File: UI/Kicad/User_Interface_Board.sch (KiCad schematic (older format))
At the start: 13 parts, among them J1 BHR-16-HUA, J2 Conn_01x02_Male, J3 Conn_01x02_Male, J4 Conn_01x02_Male, J5 Conn_01x02_Male, J6 Conn_01x08_Male, J7 Conn_01x05_Male, J8 Conn_01x03_Male

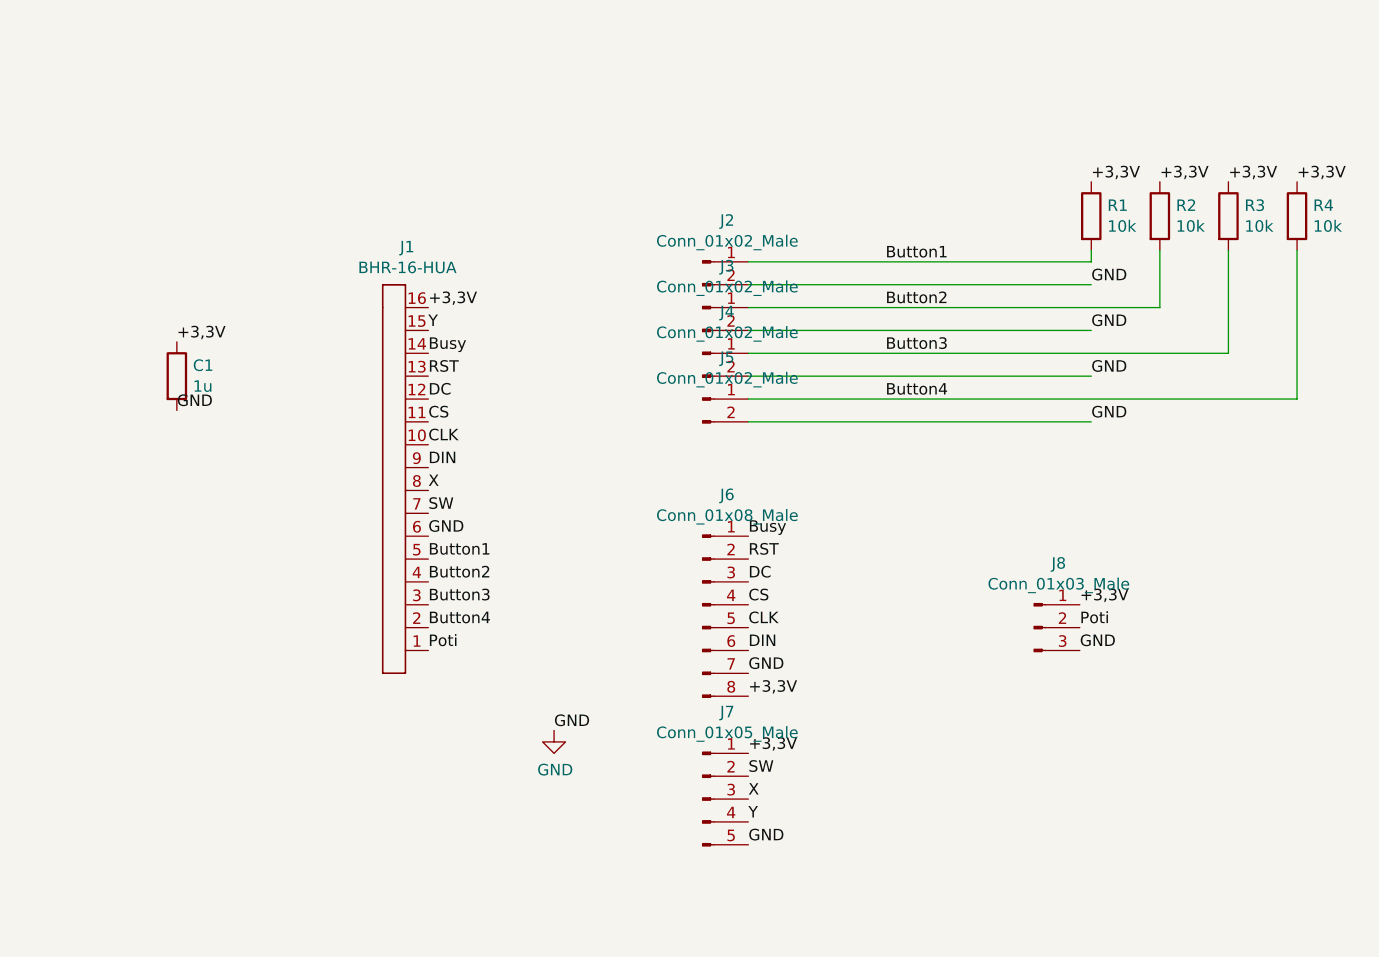
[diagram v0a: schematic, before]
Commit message: Display-Board Updated!
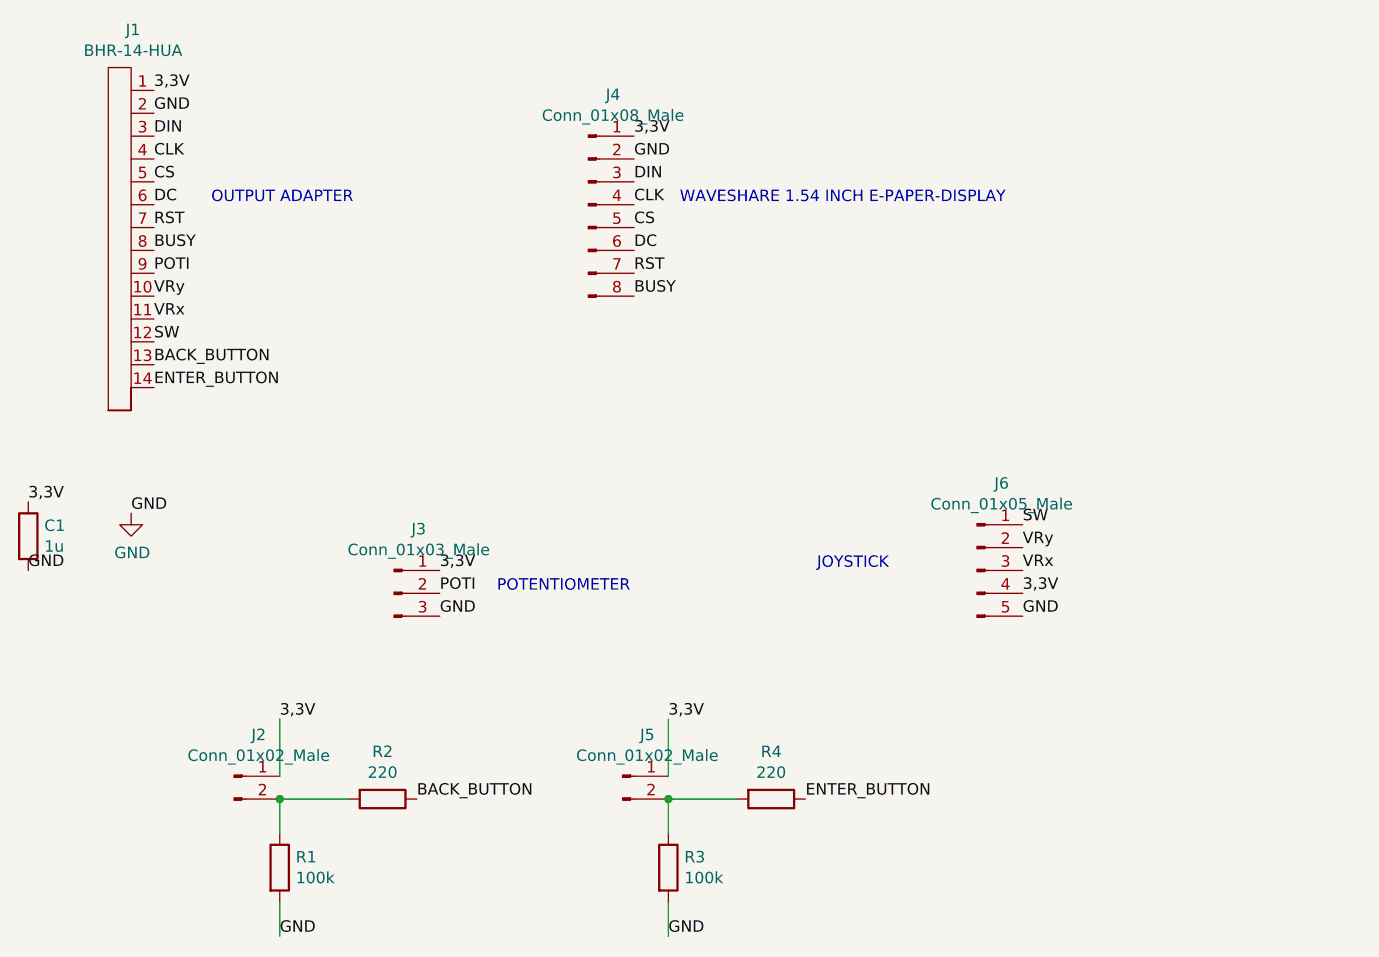
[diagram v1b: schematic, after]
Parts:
- removed J1: BHR-16-HUA, User_Interface_Board:BHR-16-HUA, symbol User_Interface_Board-rescue:BHR-16-HUA-SelfdefinedParts
- removed J3, J4, J5: Conn_01x02_Male, Connector_PinHeader_2.54mm:PinHeader_1x02_P2.54mm_Vertical, symbol Connector:Conn_01x02_Male
- added J1: BHR-14-HUA, User_Interface_Board:BHR-14-HUA, symbol User_Interface_Board-rescue:BHR-14-HUA
- added J2: Conn_01x02_Male, Connector_PinHeader_2.54mm:PinHeader_1x02_P2.54mm_Vertical, symbol Connector:Conn_01x02_Male
- C1: footprint Resistor_SMD:R_0805_2012Metric_Pad1.15x1.40mm_HandSolder -> Capacitor_SMD:C_0805_2012Metric
- R1, R3: value 10k -> 100k; footprint Resistor_SMD:R_0805_2012Metric_Pad1.15x1.40mm_HandSolder -> Resistor_SMD:R_0805_2012Metric
- R2, R4: value 10k -> 220; footprint Resistor_SMD:R_0805_2012Metric_Pad1.15x1.40mm_HandSolder -> Resistor_SMD:R_0805_2012Metric
- renumbered J8 to J3, J6 to J4, J2 to J5, J7 to J6
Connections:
- net Button3 is gone; now on net GND: R3.2
- net Y is gone; now on net 3,3V: J6.4 (Pin_4)
- net CLK: now also J4.4 (Pin_4), J1.4; no longer J4.5 (Pin_5)
- net CS: now also J4.5 (Pin_5), J1.5; no longer J4.4 (Pin_4)
- net DC: now also J4.6 (Pin_6), J1.6; no longer J4.3 (Pin_3)
- net DIN: now also J4.3 (Pin_3), J1.3; no longer J4.6 (Pin_6)
- net GND: now also J4.2 (Pin_2), R1.2, J1.2; no longer J4.7 (Pin_7), J5.2 (Pin_2)
- net RST: now also J4.7 (Pin_7), J1.7; no longer J4.2 (Pin_2)
- net SW: now also J6.1 (Pin_1), J1.12; no longer J6.2 (Pin_2)
- removed net +3,3V: C1.1, J3.1 (Pin_1), J4.8 (Pin_8), J6.1 (Pin_1), R1.1, R2.1, R3.1, R4.1
- net Busy renamed 3,3V
- net 3,3V: now also C1.1, J3.1 (Pin_1), J5.1 (Pin_1), J1.1, J2.1 (Pin_1)
- removed net Button1: J5.1 (Pin_1), R1.2
- net Button2: no longer names the net of R2.2
- net Button2: now also R1.1, J2.2 (Pin_2)
- net Button4: no longer names the net of R4.2
- net Button4: now also J5.2 (Pin_2), R3.1
- net Poti renamed POTI
- net POTI: now also J1.9
- net X renamed VRx
- net VRx: now also J1.11
- new net BACK_BUTTON: J1.13, R2.1
- new net BUSY: J1.8, J4.8 (Pin_8)
- new net ENTER_BUTTON: J1.14, R4.1
- new net VRy: J1.10, J6.2 (Pin_2)
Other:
- note added: "JOYSTICK"
- note added: "OUTPUT ADAPTER"
- note added: "POTENTIOMETER"
- note added: "WAVESHARE 1.54 INCH E-PAPER-DISPLAY"
- moved on the sheet: C1, J3, J4, J5, J6
